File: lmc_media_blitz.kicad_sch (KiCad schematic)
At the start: 31 parts, among them J3 Conn_ARM_JTAG_SWD_10, Q1 BSS138, Q2 BSS138, U1 TPS61222DCK, U2 TLV77333PDBVR, U3 LPC804M101JDH20

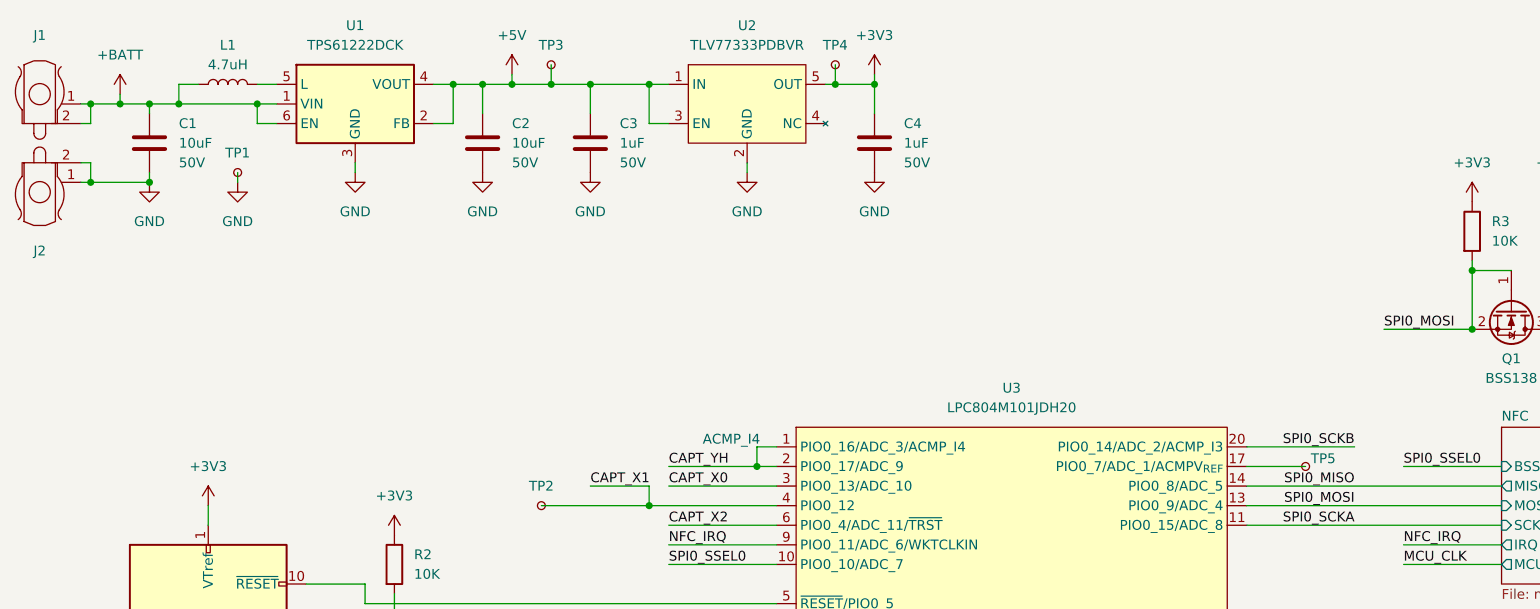
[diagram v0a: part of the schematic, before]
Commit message: Added more
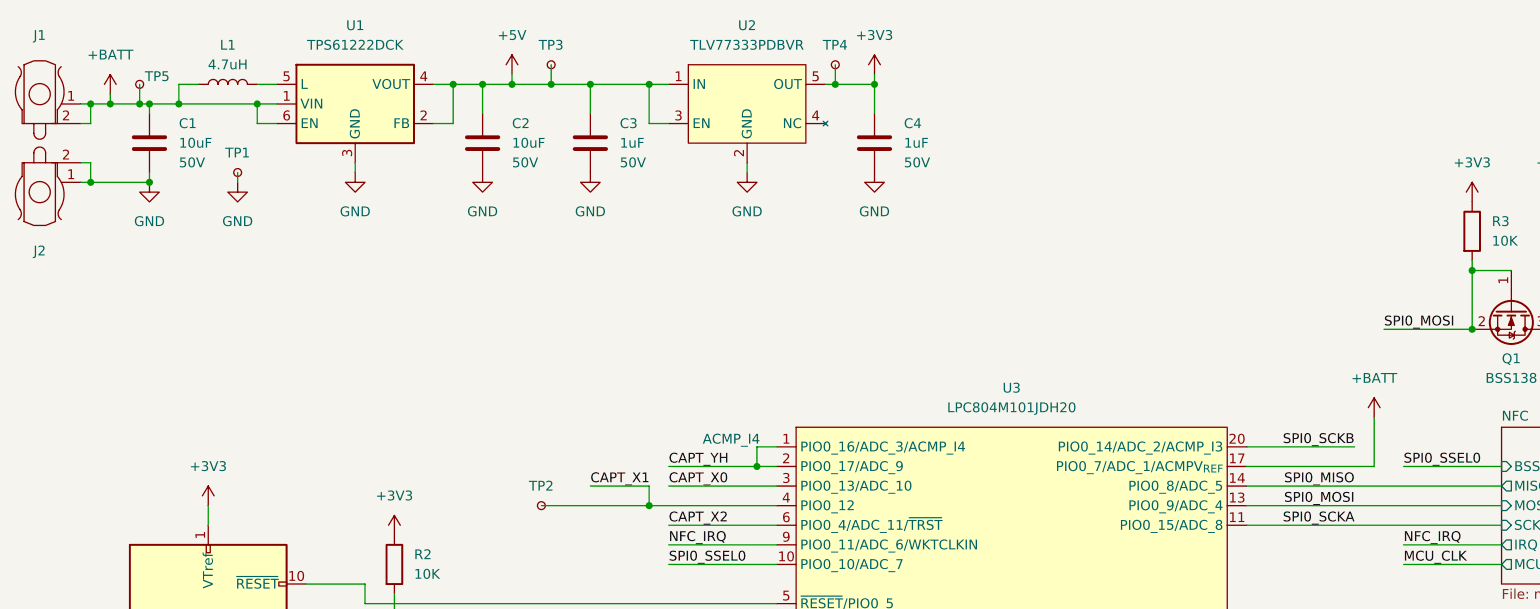
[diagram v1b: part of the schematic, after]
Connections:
- net +BATT: now also TP5.1, U3.17 (PIO0_7/ADC_1/ACMPV_{REF})
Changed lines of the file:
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@@
 	)
 	(junction
-		(at 33.02 30.48)
+		(at 35.56 30.48)
 		(diameter 0)
 		(color 0 0 0 0)
@@
 	)
 	(junction
+		(at 31.75 30.48)
+		(diameter 0)
+		(color 0 0 0 0)
+	)
+	(junction
 		(at 208.28 59.69)
 		(diameter 0)
@@
 	(wire
 		(pts
+			(xy 31.75 30.48) (xy 35.56 30.48)
+		)
+		(stroke
+			(width 0)
+			(type default)
+		)
+	)
+	(wire
+		(pts
 			(xy 88.9 25.4) (xy 88.9 27.94)
 		)
@@
 	(wire
 		(pts
+			(xy 36.83 30.48) (xy 40.64 30.48)
+		)
+		(stroke
+			(width 0)
+			(type default)
+		)
+	)
+	(wire
+		(pts
 			(xy 218.44 50.8) (xy 218.44 59.69)
 		)
@@
 	(wire
 		(pts
+			(xy 195.58 71.12) (xy 195.58 77.47)
+		)
+		(stroke
+			(width 0)
+			(type default)
+		)
+	)
+	(wire
+		(pts
 			(xy 195.58 123.19) (xy 207.01 123.19)
 		)
@@
 	(wire
 		(pts
-			(xy 179.07 77.47) (xy 186.69 77.47)
+			(xy 179.07 77.47) (xy 195.58 77.47)
 		)
 		(stroke
@@
 	(wire
 		(pts
-			(xy 33.02 30.48) (xy 33.02 29.21)
+			(xy 31.75 30.48) (xy 31.75 29.21)
 		)
 		(stroke
@@
 	(wire
 		(pts
+			(xy 35.56 27.94) (xy 35.56 30.48)
+		)
+		(stroke
+			(width 0)
+			(type default)
+		)
+	)
+	(wire
+		(pts
 			(xy 115.57 77.47) (xy 118.11 77.47)
 		)
@@
 	(wire
 		(pts
-			(xy 29.21 30.48) (xy 33.02 30.48)
+			(xy 29.21 30.48) (xy 31.75 30.48)
 		)
 		(stroke
@@
 	(wire
 		(pts
-			(xy 36.83 30.48) (xy 33.02 30.48)
+			(xy 36.83 30.48) (xy 35.56 30.48)
 		)
 		(stroke
@@
 	(wire
 		(pts
-			(xy 40.64 30.48) (xy 36.83 30.48)
-		)
-		(stroke
-			(width 0)
-			(type default)
-		)
-	)
-	(wire
-		(pts
 			(xy 44.45 116.84) (xy 44.45 118.11)
 		)
@@
 	(symbol
 		(lib_id "power:+BATT")
-		(at 33.02 29.21 0)
+		(at 31.75 29.21 0)
 		(unit 1)
 		(exclude_from_sim no)
@@
 		(fields_autoplaced yes)
 		(property "Reference" "#PWR04"
-			(at 33.02 33.02 0)
+			(at 31.75 33.02 0)
 			(effects
 				(font
@@
 		)
 		(property "Value" "+BATT"
-			(at 33.02 24.13 0)
+			(at 31.75 24.13 0)
 			(effects
 				(font
@@
 		)
 		(property "Footprint" ""
-			(at 33.02 29.21 0)
+			(at 31.75 29.21 0)
 			(effects
 				(font
@@
 		)
 		(property "Datasheet" ""
-			(at 33.02 29.21 0)
+			(at 31.75 29.21 0)
 			(effects
 				(font
@@
 		)
 		(property "Description" "Power symbol creates a global label with name \"+BATT\""
-			(at 33.02 29.21 0)
+			(at 31.75 29.21 0)
 			(effects
 				(font
@@
 	)
 	(symbol
-		(lib_id "Connector:TestPoint_Small")
-		(at 186.69 77.47 90)
-		(unit 1)
-		(exclude_from_sim no)
-		(in_bom yes)
-		(on_board yes)
-		(dnp no)
-		(property "Reference" "TP5"
-			(at 188.976 76.454 90)
-			(effects
-				(font
-					(size 1.27 1.27)
-				)
-			)
-		)
-		(property "Value" "TestPoint_Small"
-			(at 187.9599 76.2 0)
-			(effects
-				(font
-					(size 1.27 1.27)
-				)
-				(justify left)
-				(hide yes)
-			)
-		)
-		(property "Footprint" "TestPoint:TestPoint_Pad_D2.0mm"
-			(at 186.69 72.39 0)
-			(effects
-				(font
-					(size 1.27 1.27)
-				)
-				(hide yes)
-			)
-		)
-		(property "Datasheet" "~"
-			(at 186.69 72.39 0)
-			(effects
-				(font
-					(size 1.27 1.27)
-				)
-				(hide yes)
-			)
-		)
-		(property "Description" "test point"
-			(at 186.69 77.47 0)
-			(effects
-				(font
-					(size 1.27 1.27)
-				)
-				(hide yes)
-			)
-		)
-		(pin "1"
-		)
-		(instances
-			(project "lmc_media_blitz"
-				(path "/b87eb037-3127-4116-a225-5eb939725614"
-					(reference "TP5")
-					(unit 1)
-				)
-			)
-		)
-	)
-	(symbol
 		(lib_id "Device:R")
 		(at 208.28 46.99 0)
@@
 	)
 	(symbol
+		(lib_id "Connector:TestPoint_Small")
+		(at 35.56 27.94 90)
+		(unit 1)
+		(exclude_from_sim no)
+		(in_bom yes)
+		(on_board yes)
+		(dnp no)
+		(property "Reference" "TP5"
+			(at 37.846 26.924 90)
+			(effects
+				(font
+					(size 1.27 1.27)
+				)
+			)
+		)
+		(property "Value" "TestPoint_Small"
+			(at 36.8299 26.67 0)
+			(effects
+				(font
+					(size 1.27 1.27)
+				)
+				(justify left)
+				(hide yes)
+			)
+		)
+		(property "Footprint" "TestPoint:TestPoint_Pad_D2.0mm"
+			(at 35.56 22.86 0)
+			(effects
+				(font
+					(size 1.27 1.27)
+				)
+				(hide yes)
+			)
+		)
+		(property "Datasheet" "~"
+			(at 35.56 22.86 0)
+			(effects
+				(font
+					(size 1.27 1.27)
+				)
+				(hide yes)
+			)
+		)
+		(property "Description" "test point"
+			(at 35.56 27.94 0)
+			(effects
+				(font
+					(size 1.27 1.27)
+				)
+				(hide yes)
+			)
+		)
+		(pin "1"
+		)
+		(instances
+			(project "lmc_media_blitz"
+				(path "/b87eb037-3127-4116-a225-5eb939725614"
+					(reference "TP5")
+					(unit 1)
+				)
+			)
+		)
+	)
+	(symbol
 		(lib_id "power:GND")
 		(at 44.45 118.11 0)
@@
 					(unit 1)
 				)
+			)
+		)
+	)
+	(symbol
+		(lib_id "power:+BATT")
+		(at 195.58 71.12 0)
+		(unit 1)
+		(exclude_from_sim no)
+		(in_bom yes)
+		(on_board yes)
+		(dnp no)
+		(fields_autoplaced yes)
+		(property "Reference" "#PWR063"
+			(at 195.58 74.93 0)
+			(effects
+				(font
+					(size 1.27 1.27)
+				)
+				(hide yes)
+			)
+		)
+		(property "Value" "+BATT"
+			(at 195.58 66.04 0)
+			(effects
+				(font
+					(size 1.27 1.27)
+				)
+			)
+		)
+		(property "Footprint" ""
+			(at 195.58 71.12 0)
+			(effects
+				(font
+					(size 1.27 1.27)
+				)
+				(hide yes)
+			)
+		)
+		(property "Datasheet" ""
+			(at 195.58 71.12 0)
+			(effects
+				(font
+					(size 1.27 1.27)
+				)
+				(hide yes)
+			)
+		)
+		(property "Description" "Power symbol creates a global label with name \"+BATT\""
+			(at 195.58 71.12 0)
+			(effects
+				(font
+					(size 1.27 1.27)
+				)
+				(hide yes)
+			)
+		)
+		(pin "1"
+		)
+		(instances
+			(project "lmc_media_blitz"
+				(path "/b87eb037-3127-4116-a225-5eb939725614"
+					(reference "#PWR063")
+					(unit 1)
+				)
